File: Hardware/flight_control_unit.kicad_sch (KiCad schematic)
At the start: 36 parts, among them SW3 SW_SPDT, SW4 SW_Push_Dual, U12 STM32F405RGTx, Y2 25MHz

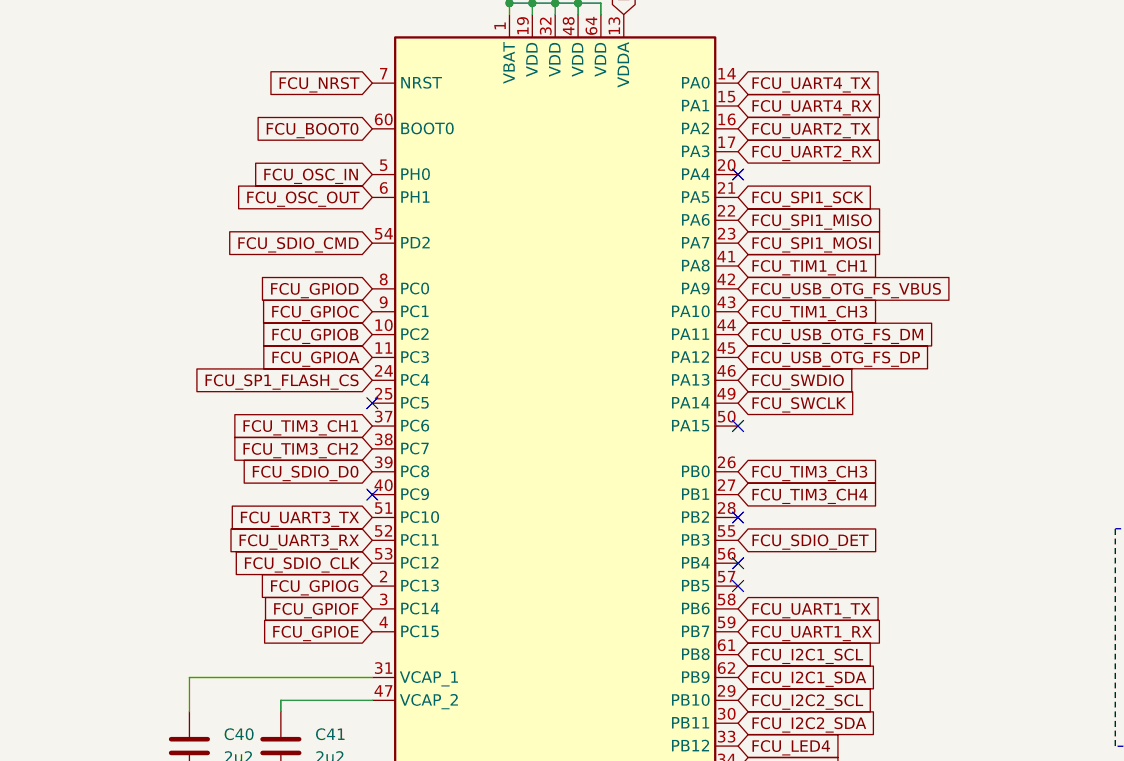
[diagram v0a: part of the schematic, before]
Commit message: pin refatoration, freertos code
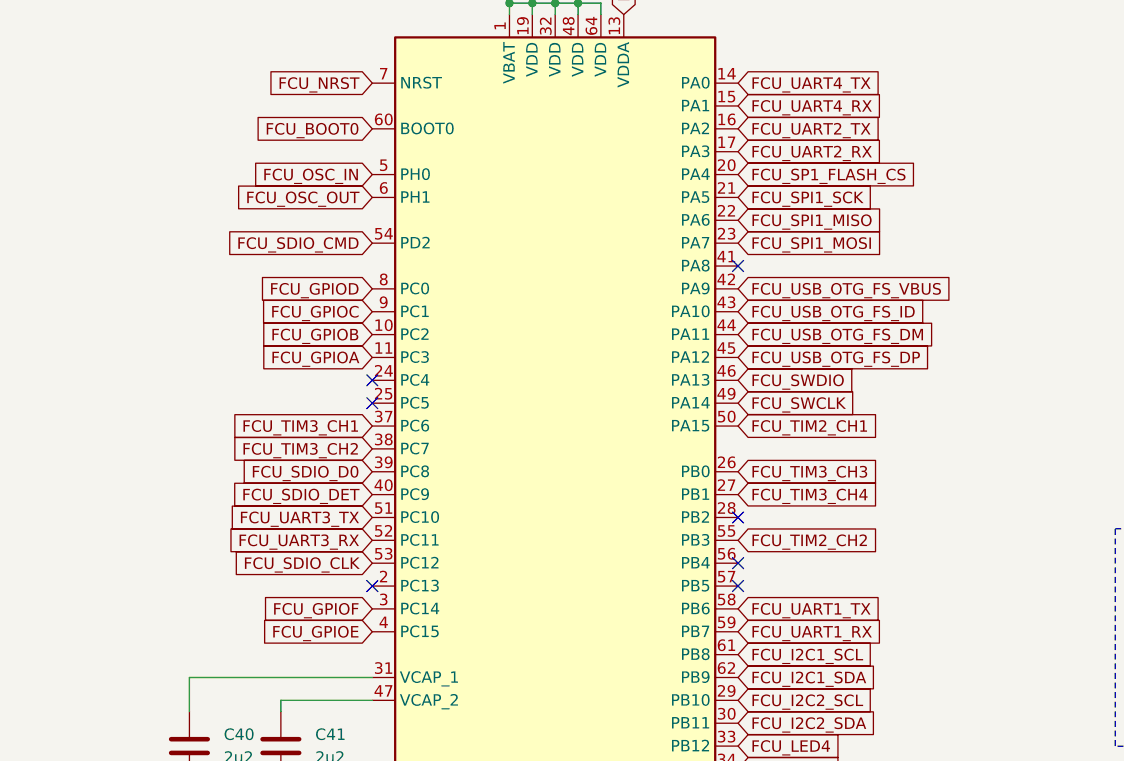
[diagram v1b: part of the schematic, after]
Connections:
- net FCU_SDIO_DET: now also U12.40 (PC9); no longer U12.55 (PB3)
- net FCU_SP1_FLASH_CS: now also U12.20 (PA4); no longer U12.24 (PC4)
- net FCU_TIM2_CH1: now reaches U12.50 (PA15)
- net FCU_GPIOG: no longer names the net of U12.2 (PC13)
- net FCU_TIM1_CH1: no longer names the net of U12.41 (PA8)
- net FCU_TIM1_CH3 renamed FCU_USB_OTG_FS_ID
- new net FCU_TIM2_CH2: U12.55 (PB3)
